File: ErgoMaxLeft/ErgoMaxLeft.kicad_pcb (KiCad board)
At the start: 2 copper layers, 182.8 x 178.9 mm, 97 parts, among them J1 AudioJack4_Ground, K1 KEYSW, K10 KEYSW, K11 KEYSW, K12 KEYSW, K13 KEYSW, K14 KEYSW, K15 KEYSW, K16 KEYSW, K17 KEYSW, K18 KEYSW, K19 KEYSW, K2 KEYSW, K20 KEYSW, K21 KEYSW, K22 KEYSW, K23 KEYSW, K24 KEYSW, K25 KEYSW, K26 KEYSW, K27 KEYSW, K28 KEYSW, K29 KEYSW, K3 KEYSW, K30 KEYSW, K31 KEYSW, K32 KEYSW, K33 KEYSW, K34 KEYSW, K35 KEYSW, K36 KEYSW, K37 KEYSW, K38 KEYSW, K39 KEYSW, K4 KEYSW, K40 KEYSW, K41 KEYSW, K42 KEYSW, K43 KEYSW, K44 KEYSW, K5 KEYSW, K6 KEYSW, K7 KEYSW, K8 KEYSW, K9 KEYSW, U1 ProMicro

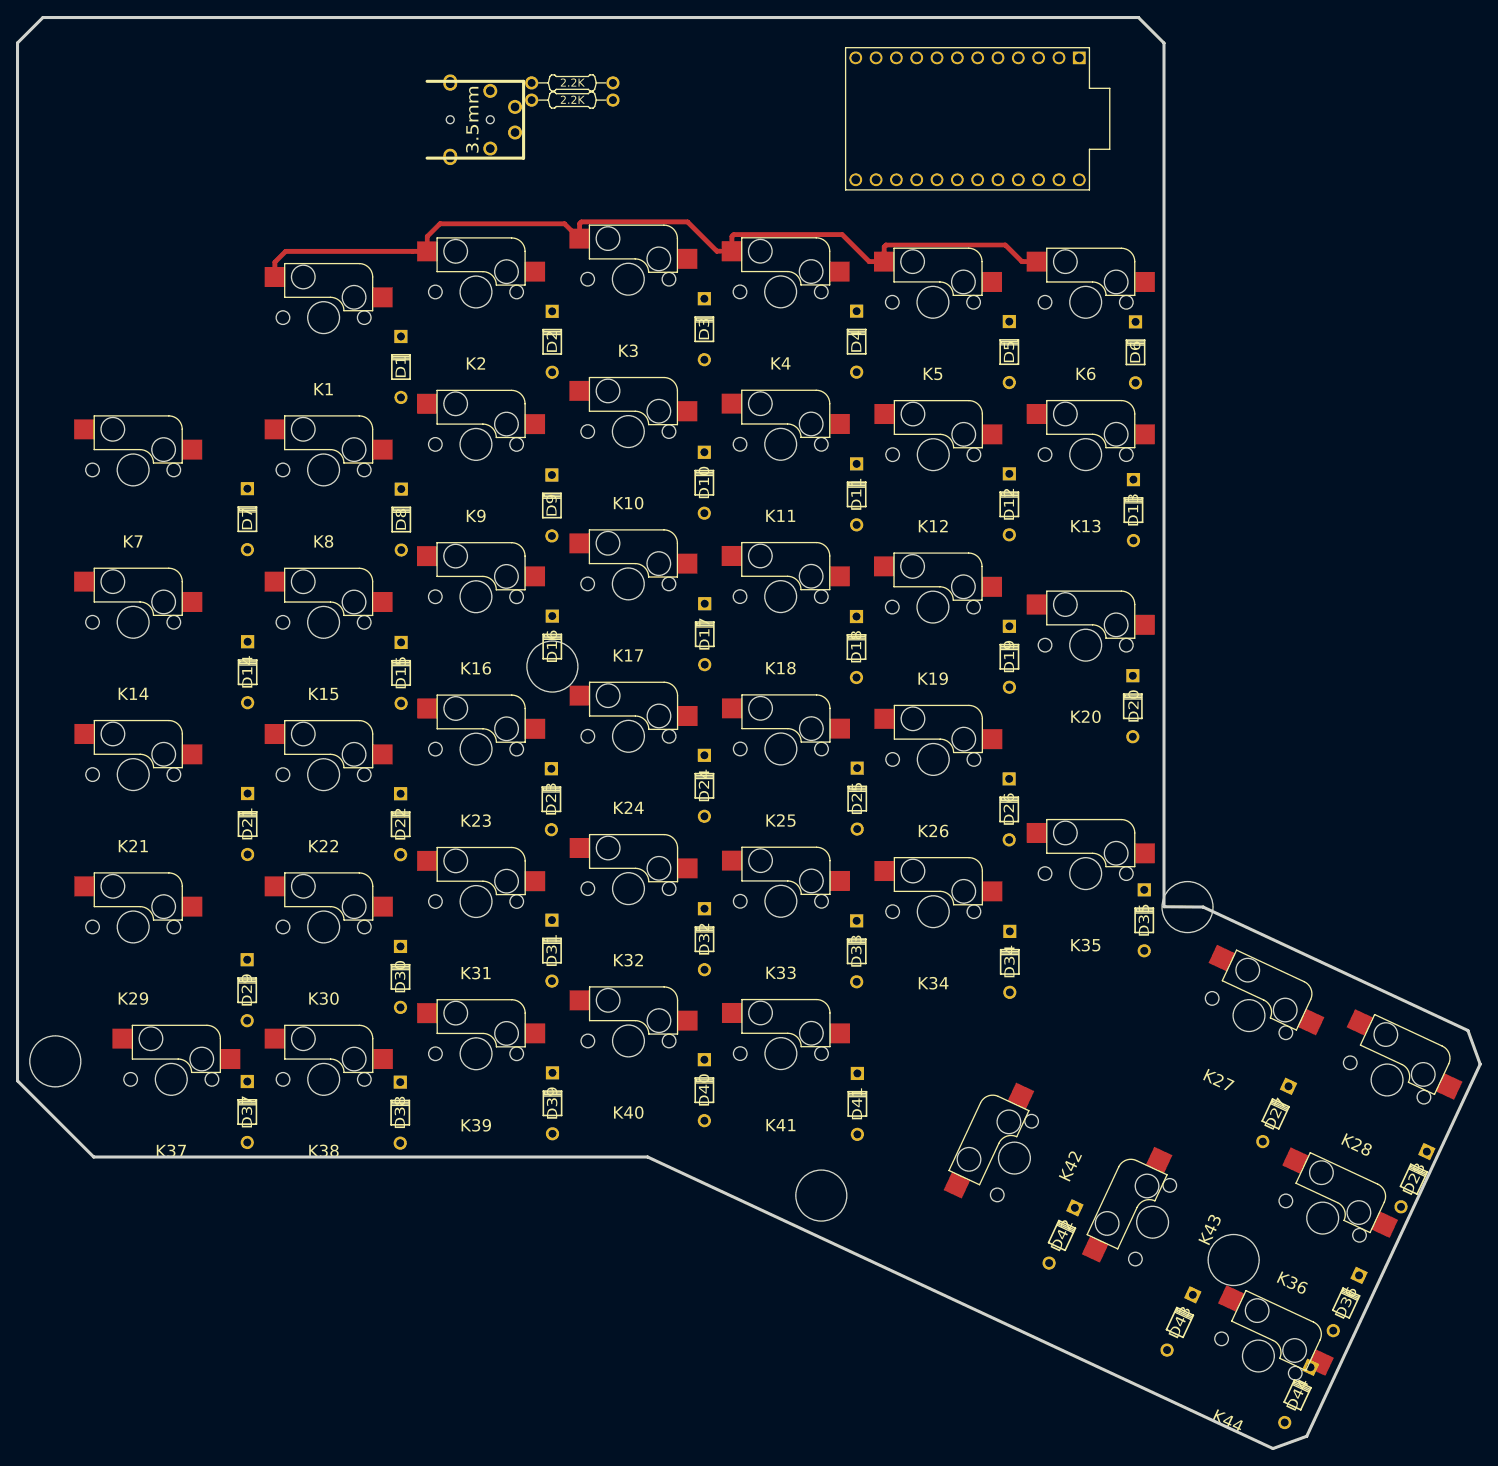
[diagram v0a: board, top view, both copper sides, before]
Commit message: WIP PCB - more routing
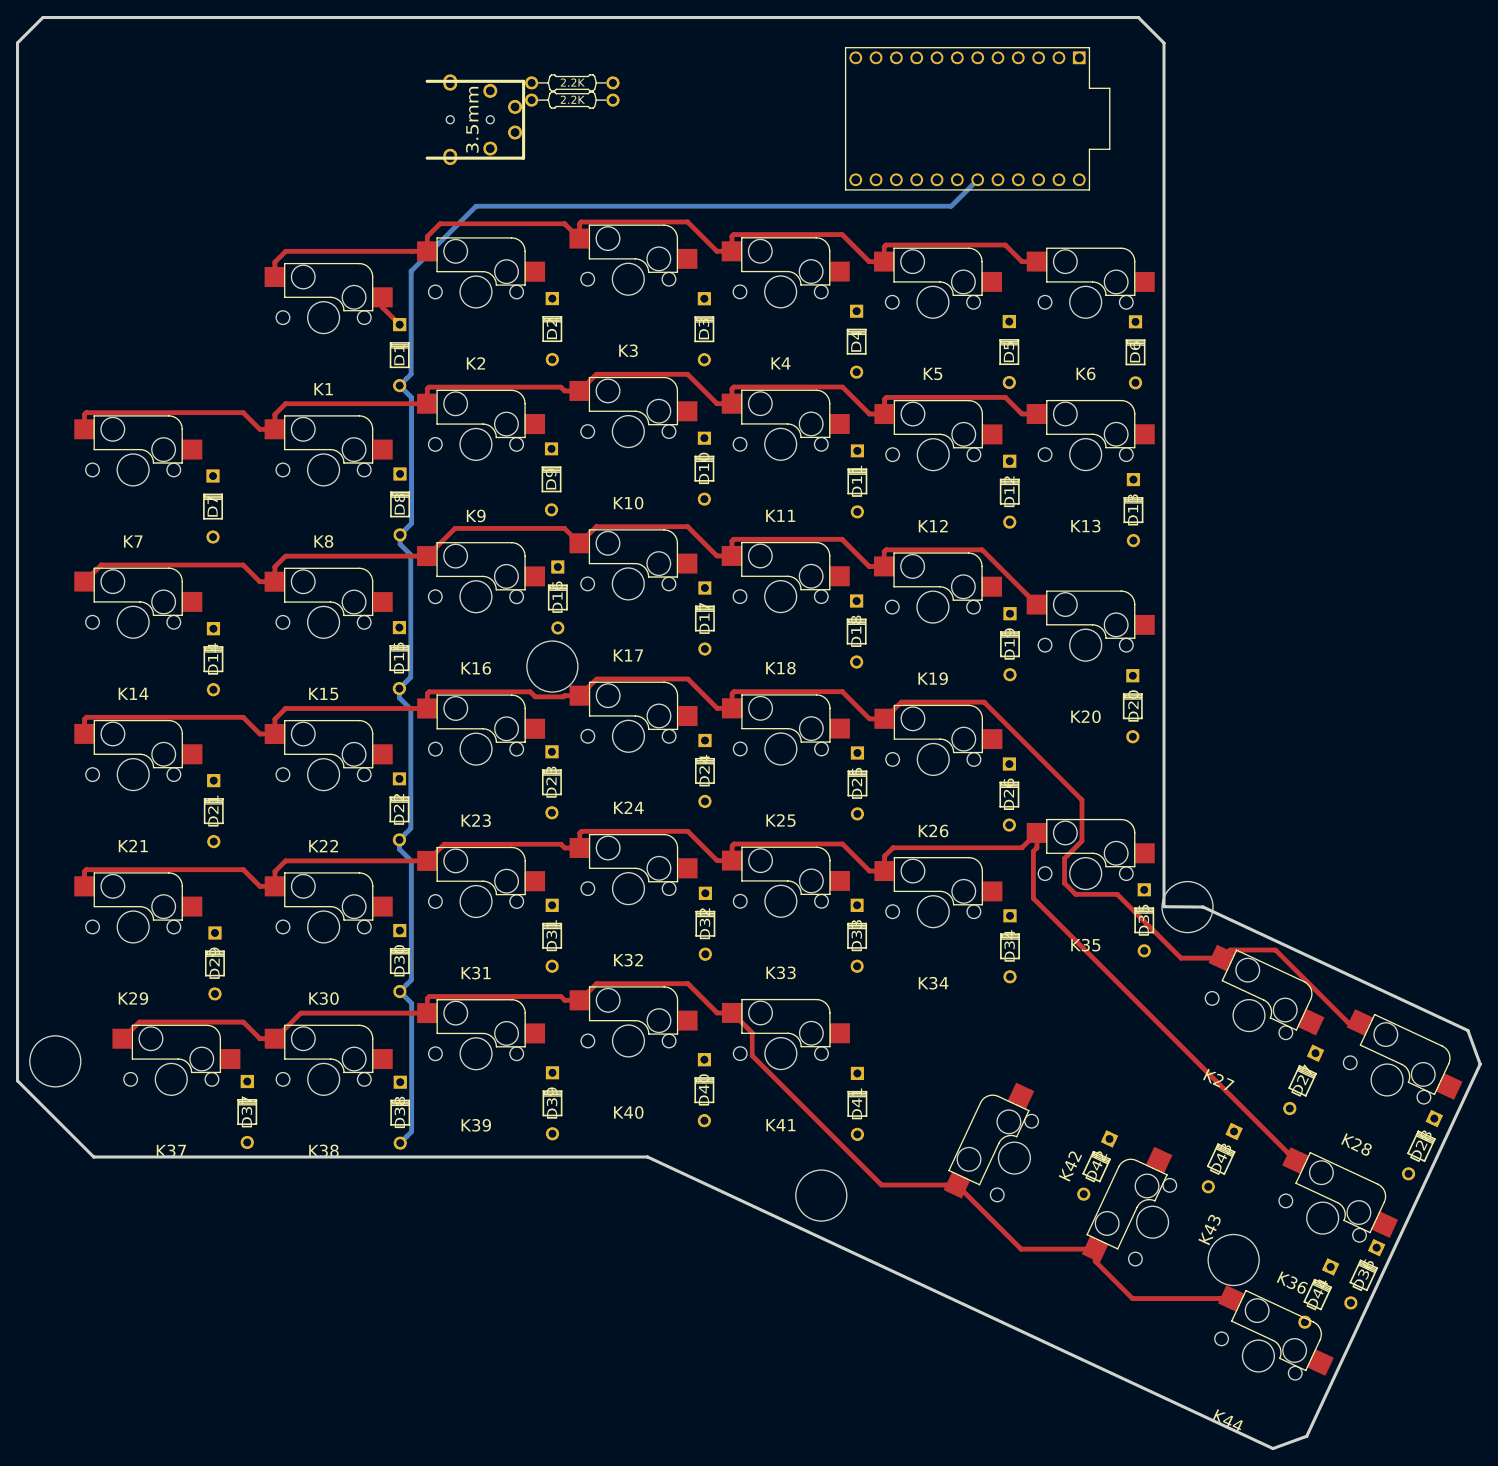
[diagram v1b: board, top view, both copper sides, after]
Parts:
- moved D43 21.1 mm to (260.8, 168.8)
- moved D44 12.8 mm to (272.9, 185.8)
- moved D42 9.64 mm to (245.2, 169.8)
- moved D16 6.18 mm to (177.9, 98.6)
- moved D27 5.33 mm to (271.0, 159.1)
- moved D29 5.24 mm to (135.0, 144.4)
- moved D7 4.57 mm to (134.8, 87.3)
- moved D14 4.57 mm to (134.8, 106.3)
- moved D21 4.53 mm to (134.9, 125.3)
- moved D28 4.23 mm to (285.8, 167.2)
- moved D36 4.11 mm to (278.6, 183.4)
- moved D9 3.27 mm to (177.1, 83.9)
- moved D23 2.11 mm to (177.1, 121.7)
- moved D30 1.98 mm to (158.1, 144.1)
- moved D17 1.96 mm to (196.3, 101.3)
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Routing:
- net /Row3: track 0.00 -> 200.1 mm
- net /Col1: track 0.00 -> 191.1 mm
- net /Row4: track 0.00 -> 189.9 mm
- net /Row5: track 0.00 -> 163.5 mm
- net /Row2: track 0.00 -> 135.9 mm
- net /Row1: track 0.00 -> 135.0 mm
- net Net-(D1-Pad2): track 0.00 -> 4.31 mm
